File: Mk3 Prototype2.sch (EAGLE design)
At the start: 142 parts, among them IC1 TPD3E001DRL, IC2 TPS62082, IC3 STM32F401V, IC4 BQ2409X, IC6 CC3100MOD, IC7 BQ2970, J1 ZX62-AB-5PA(11), J2 ER-TFT024-3, J3 SWD_SHROUD, Q1 DMMT5401, Q2 CSD25402Q3A, Q3 CSD13202Q2, Q4 CSD85301Q2, Q6 CSD25402Q3A, Q8 CSD13202Q2, SW1 JOYSTICK_MINI_MULTICOMP, U1 USD-SOCKET-SDIODM3AT_0011, X2 16MHz-3.2-2.5, X3 ABS07-32.768KHZ-T

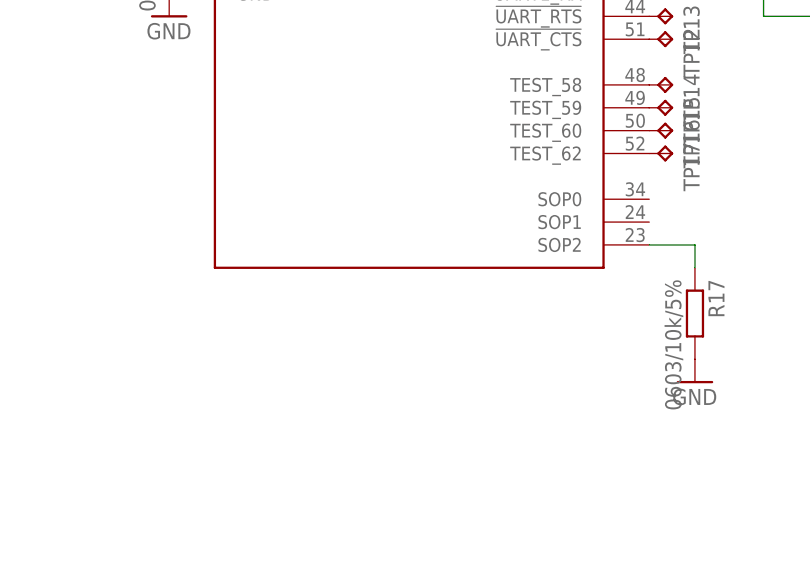
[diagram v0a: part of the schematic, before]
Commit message: moving things around
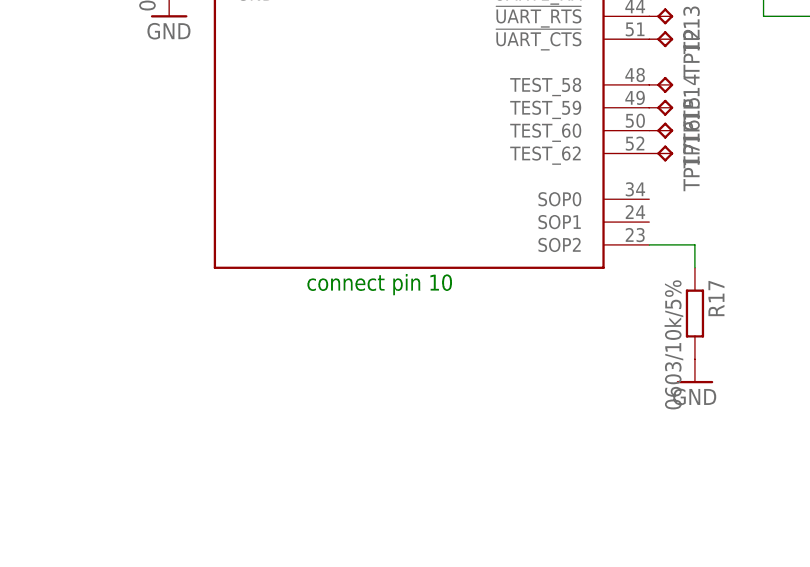
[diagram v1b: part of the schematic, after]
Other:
- note added: "connect pin 10"
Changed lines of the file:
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@@
 <text x="162.56" y="106.68" size="1.778" layer="91">needed?</text>
 <text x="414.02" y="50.8" size="1.778" layer="91">change footprint once final part is known</text>
+<text x="693.42" y="160.02" size="1.778" layer="91">connect pin 10</text>
 </plain>
 <instances>
